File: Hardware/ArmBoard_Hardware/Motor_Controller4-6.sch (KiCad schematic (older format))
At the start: 18 parts, among them U10 LTC6900, U11 LTC6900, U12 TB67H400AFNG,EL, U13 TB67H400AFNG,EL, U14 LTC6900, U15 TB67H400AFNG,EL

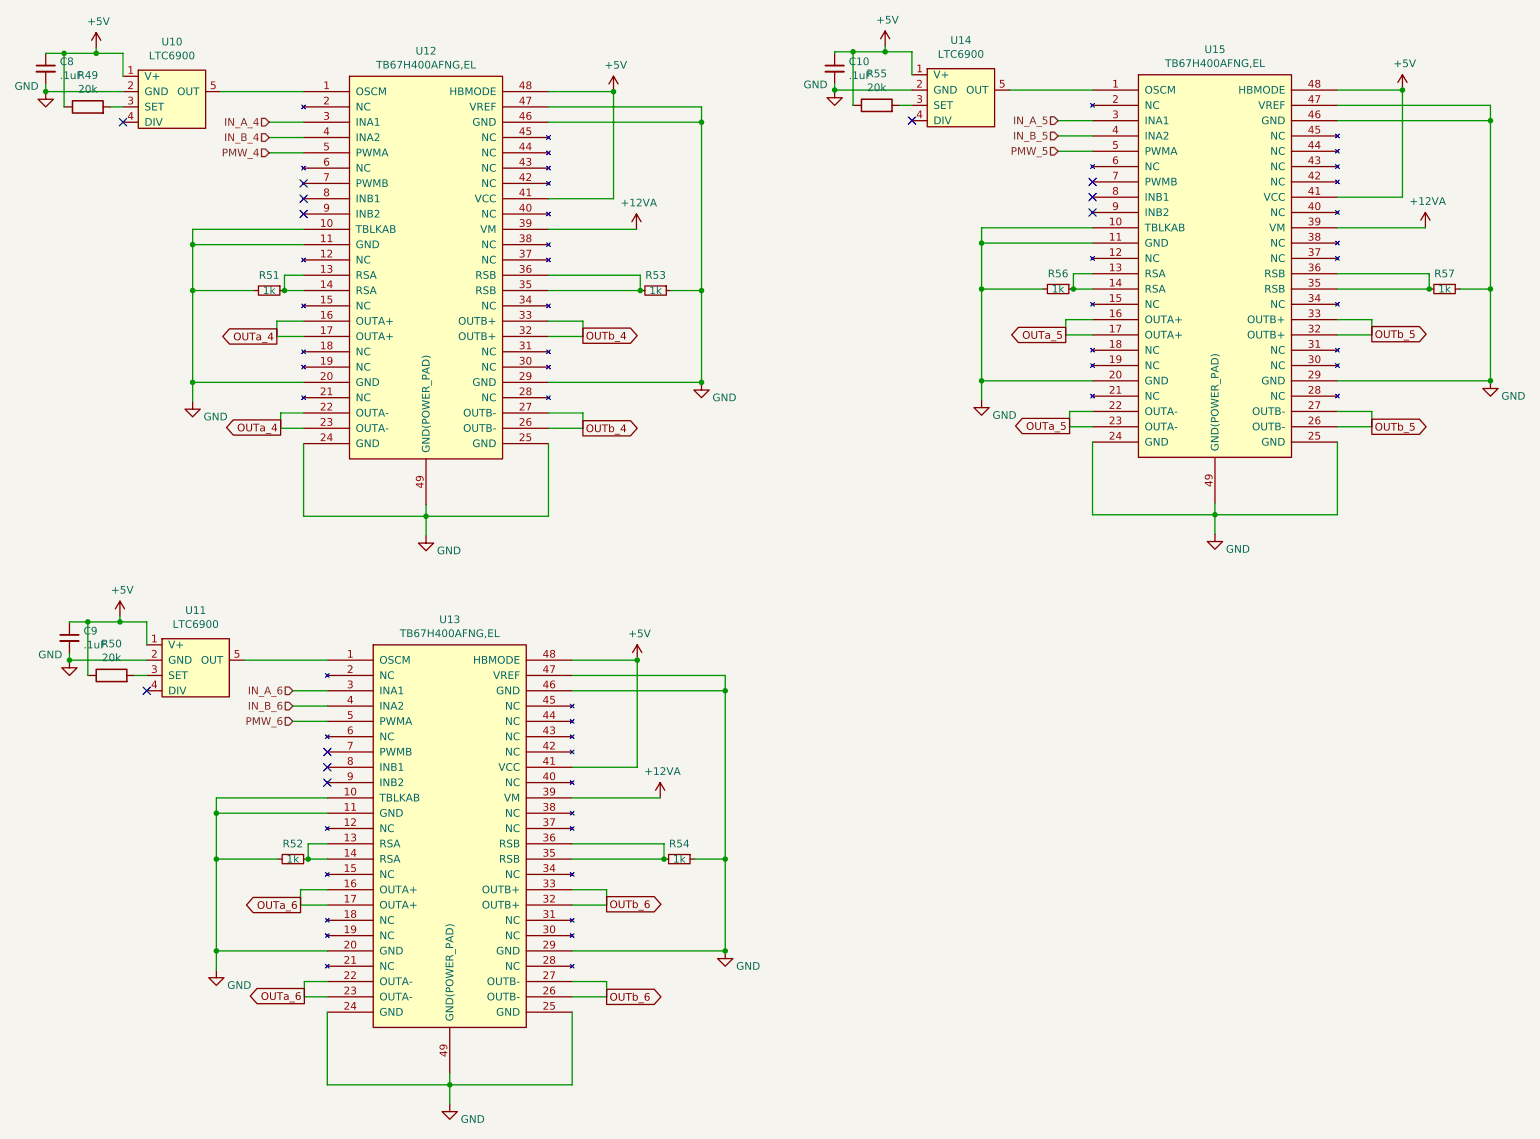
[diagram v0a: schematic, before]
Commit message: armboard review
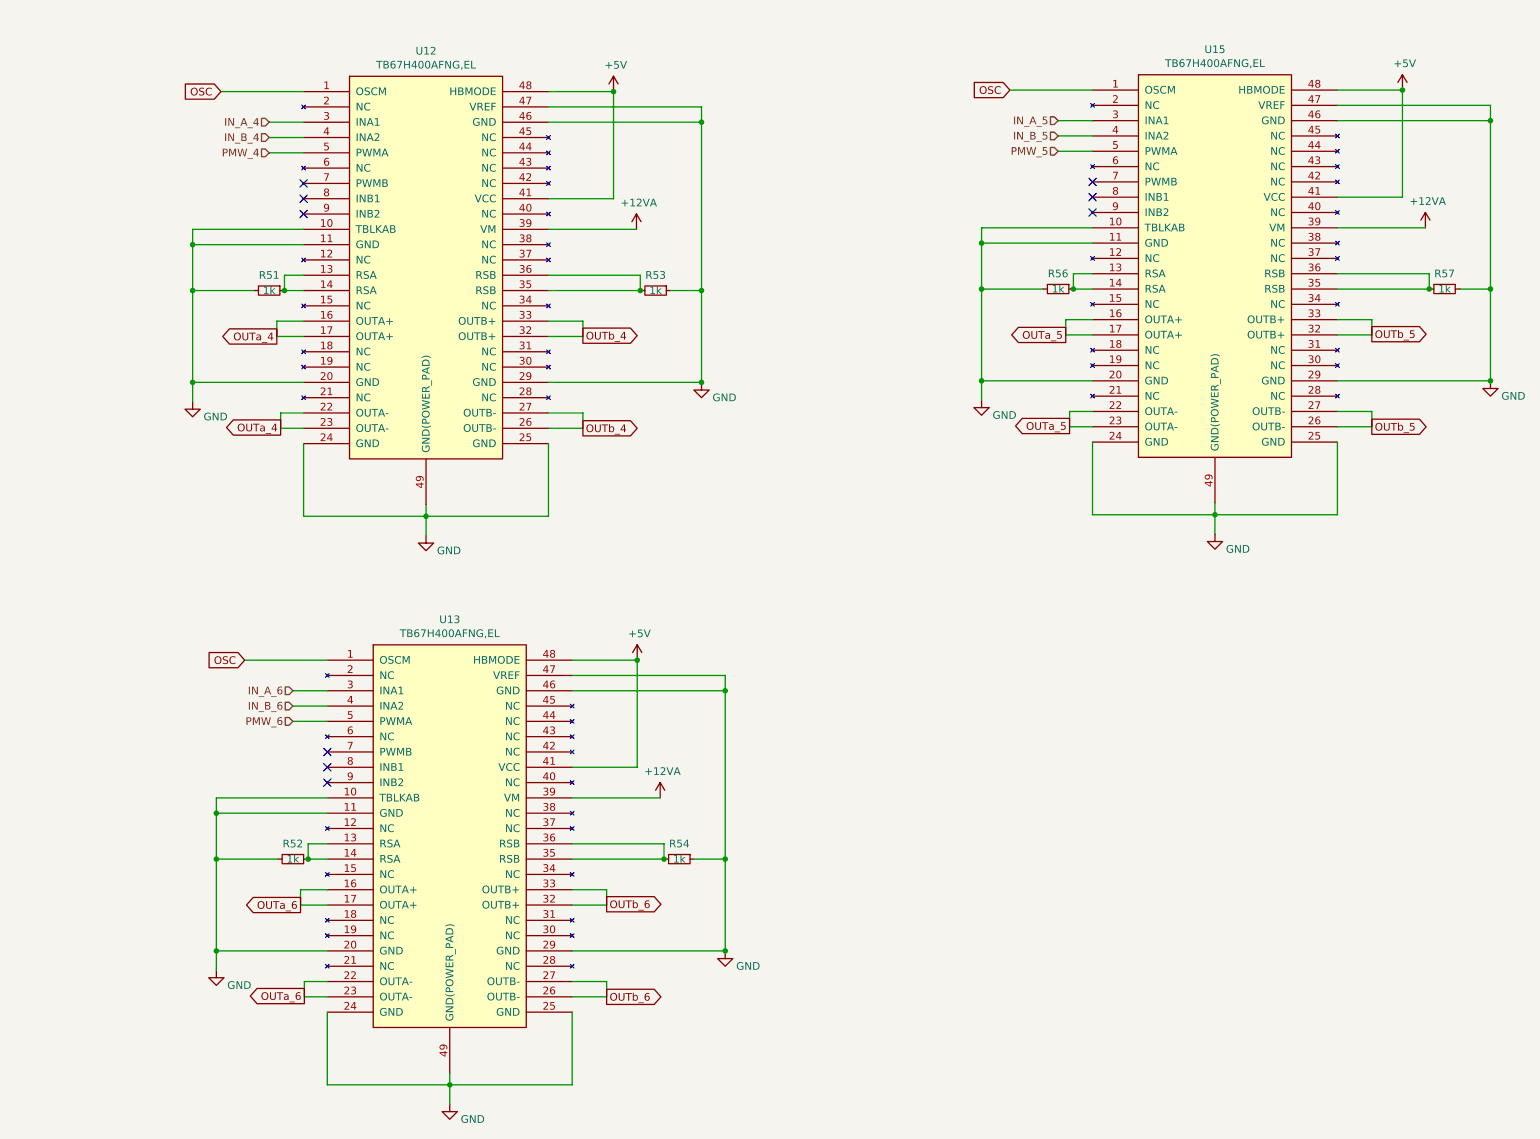
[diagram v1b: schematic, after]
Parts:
- removed C10, C8, C9: .1uF, Capacitor_SMD:C_0603_1608Metric_Pad1.08x0.95mm_HandSolder, symbol Device:C_Small
- removed R49, R50, R55: 20k, Resistor_SMD:R_0603_1608Metric_Pad0.98x0.95mm_HandSolder, symbol Device:R
- removed U10, U11, U14: LTC6900, Package_TO_SOT_SMD:SOT-23-5_HandSoldering, symbol ArmBoard_Hardware-rescue:LTC6900-MRDT_Devices
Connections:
- net OSC: now reaches U12.1 (OSCM)
- net OSC: now also U13.1 (OSCM), U15.1 (OSCM)
- no-connect marks 12 -> 9

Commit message: Rescued the Libaries
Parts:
- U12, U13, U15: symbol ArmBoard_Hardware-rescue:TB67H400AFNG,EL-MRDT_ICs -> MRDT_ICs:TB67H400AFNG,EL
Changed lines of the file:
@@
 IN_A_4
 $Comp
-L ArmBoard_Hardware-rescue:TB67H400AFNG,EL-MRDT_ICs U?
+L MRDT_ICs:TB67H400AFNG,EL U?
 U 1 1 624C6CB1
 P 3160 2365
 AR Path="/63845F20/624C6CB1" Ref="U?"  Part="1"
 AR Path="/63845FEF/624C6CB1" Ref="U12"  Part="1"
+AR Path="/624C6CB1" Ref="U12"  Part="1"
 F 0 "U12" H 3160 3980 50  0000 C CNN
 F 1 "TB67H400AFNG,EL" H 3160 3889 50  0000 C CNN
@@
 	8315 3905 8315 3780
 $Comp
-L ArmBoard_Hardware-rescue:TB67H400AFNG,EL-MRDT_ICs U?
+L MRDT_ICs:TB67H400AFNG,EL U?
 U 1 1 6250A1E6
 P 8315 2355
 AR Path="/63845F20/6250A1E6" Ref="U?"  Part="1"
 AR Path="/63845FEF/6250A1E6" Ref="U15"  Part="1"
+AR Path="/6250A1E6" Ref="U15"  Part="1"
 F 0 "U15" H 8315 3970 50  0000 C CNN
 F 1 "TB67H400AFNG,EL" H 8315 3879 50  0000 C CNN
@@
 	3315 7630 3315 7505
 $Comp
-L ArmBoard_Hardware-rescue:TB67H400AFNG,EL-MRDT_ICs U?
+L MRDT_ICs:TB67H400AFNG,EL U?
 U 1 1 62512CF8
 P 3315 6080
 AR Path="/63845F20/62512CF8" Ref="U?"  Part="1"
 AR Path="/63845FEF/62512CF8" Ref="U13"  Part="1"
+AR Path="/62512CF8" Ref="U13"  Part="1"
 F 0 "U13" H 3315 7695 50  0000 C CNN
 F 1 "TB67H400AFNG,EL" H 3315 7604 50  0000 C CNN
